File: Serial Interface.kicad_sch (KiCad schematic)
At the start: 34 parts, among them J23 *, J24 *, J25 *, J26 *, J27 *, J28 *, J29 *, J30 *, J31 *, J32 *, U7 *, U8 *

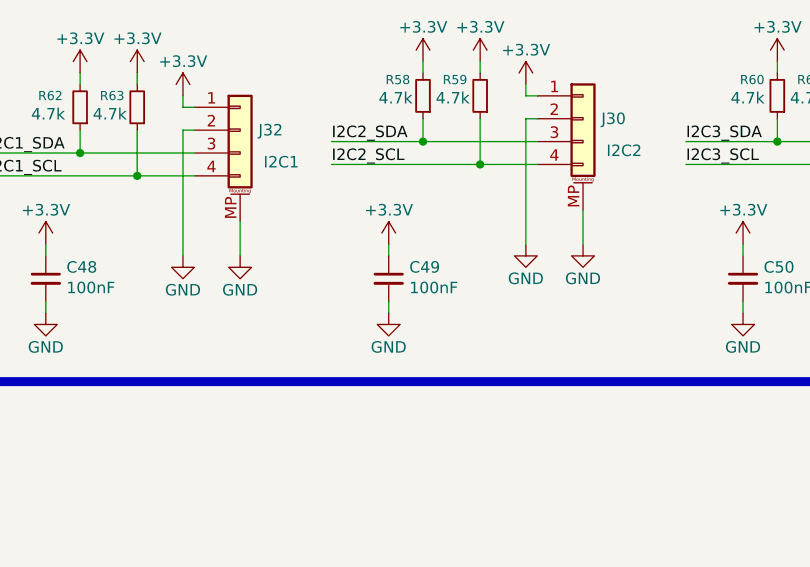
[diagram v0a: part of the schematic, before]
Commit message: [Schematic][Modify] Monification of simulation models
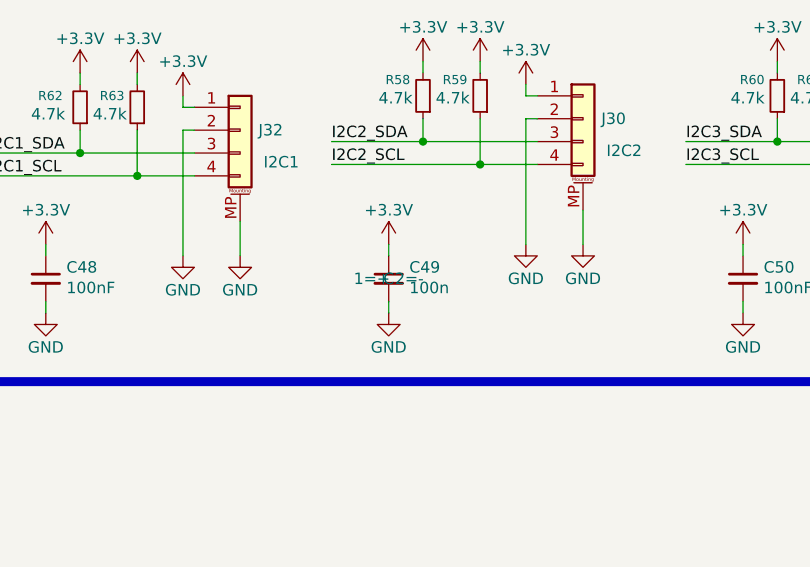
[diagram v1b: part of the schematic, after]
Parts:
- C49: value 100nF -> 100n
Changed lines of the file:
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@@
 			)
 		)
-		(property "Value" "100nF"
+		(property "Value" "100n"
 			(at 210.566 141.986 0)
 			(effects
@@
 			)
 		)
+		(property "Sim.Device" "C"
+			(at 208.28 140.97 0)
+			(effects
+				(font
+					(size 1.27 1.27)
+				)
+			)
+		)
+		(property "Sim.Pins" "1=+ 2=-"
+			(at 208.28 140.97 0)
+			(effects
+				(font
+					(size 1.27 1.27)
+				)
+			)
+		)
 		(pin "2"
 		)
@@
 			)
 		)
+		(property "Sim.Library" ".\\"
+			(at 54.61 66.04 0)
+			(effects
+				(font
+					(size 1.27 1.27)
+				)
+				(hide yes)
+			)
+		)
 		(pin "5"
 		)
@@
 			(at 207.01 66.04 0)
 			(effects
+				(font
+					(size 1.27 1.27)
+				)
+				(hide yes)
+			)
+		)
+		(property "Sim.Library" ".\\"
+			(at 207.01 66.04 0)
+			(effects
